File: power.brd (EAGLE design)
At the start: 120 x 120 mm, 34 parts, among them CN1 21700, CN2 21700, CN3 21700, CN5 15PIN 0.5MM, Q1 SIRA36DP-T1-GE3, Q2 SIRA36DP-T1-GE3, U1 MAX17320G20+

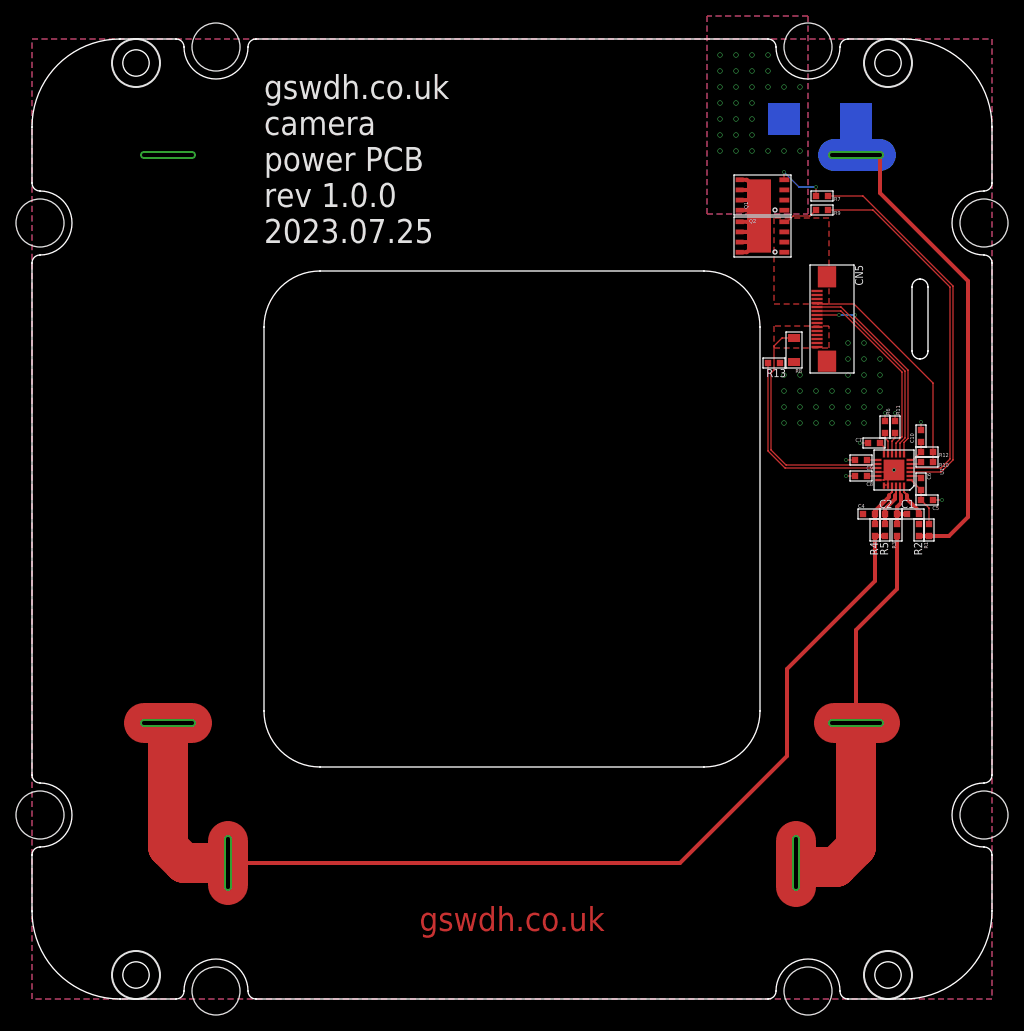
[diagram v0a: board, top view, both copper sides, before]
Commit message: MIPI length matched DRC passes
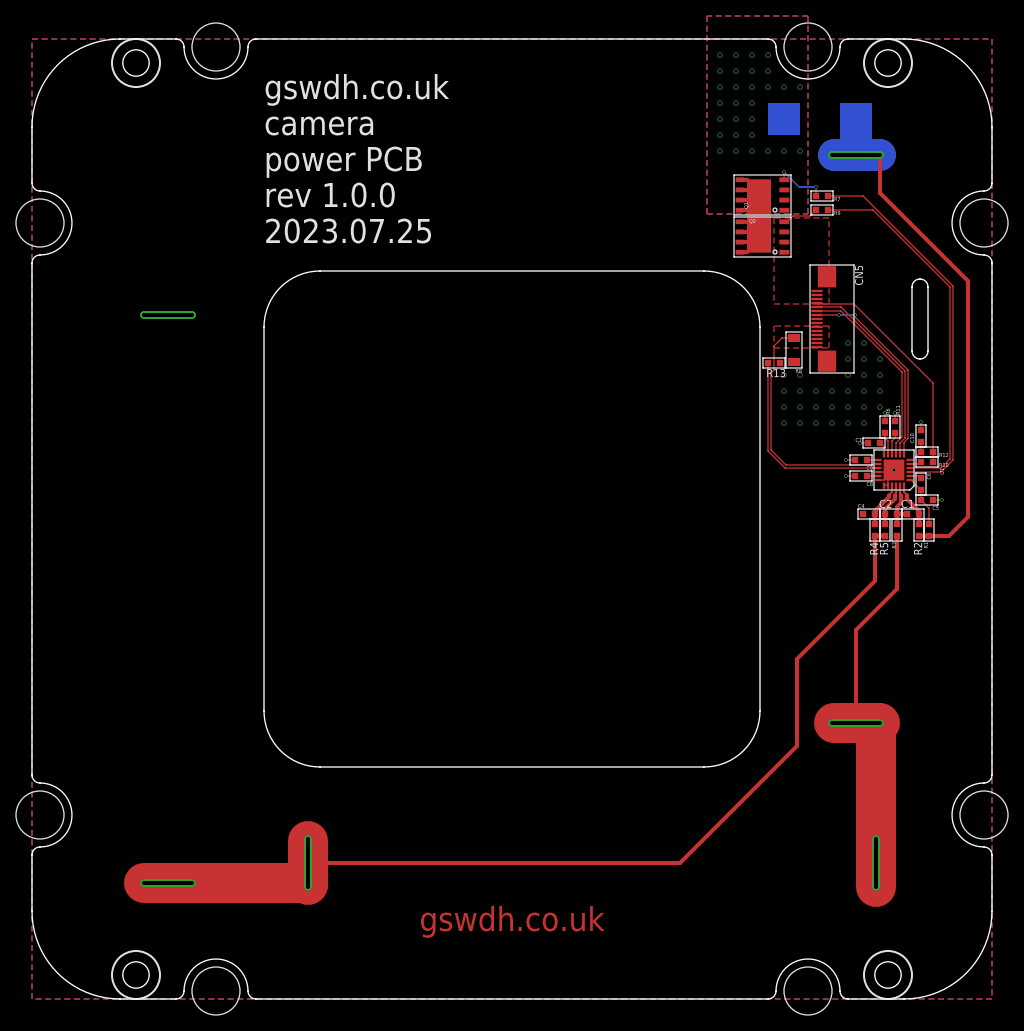
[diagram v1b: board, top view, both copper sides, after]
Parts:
- moved CN1 20.0 mm to (-43.0, -10.0)
- moved CN2 10.0 mm to (10.0, -43.0)
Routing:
- net PACK_MID: track 143.8 -> 130.0 mm
- net N$4: track 61.0 -> 57.5 mm
- net N$1: track 4.32 -> 5.57 mm
